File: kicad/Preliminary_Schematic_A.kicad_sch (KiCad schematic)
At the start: 5 parts, among them M1 Motor_Servo, U2 40PC015G, U3 TSSP58038

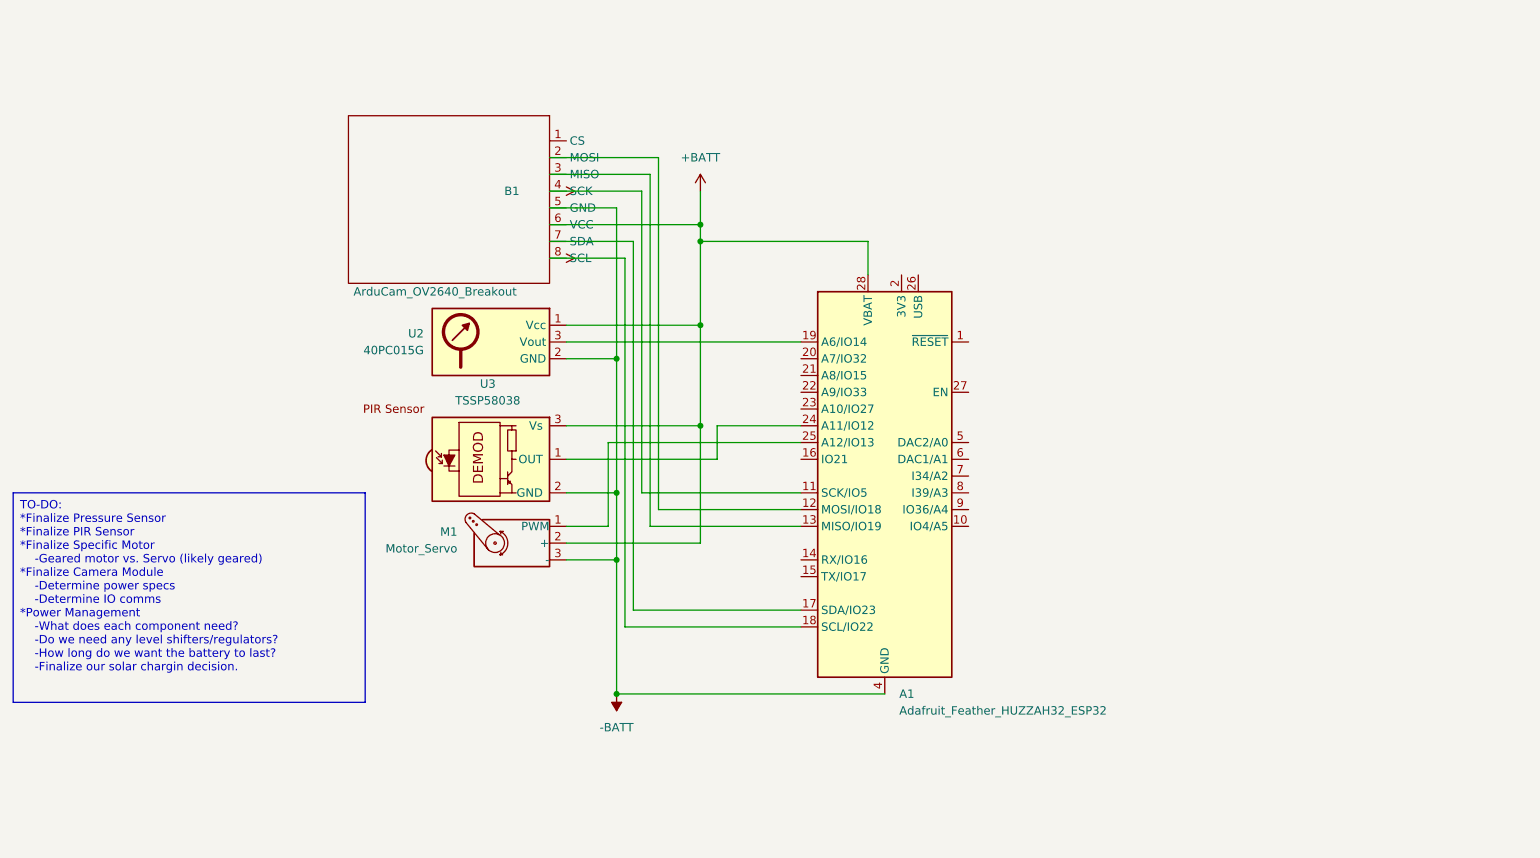
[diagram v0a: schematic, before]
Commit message: Add files via upload
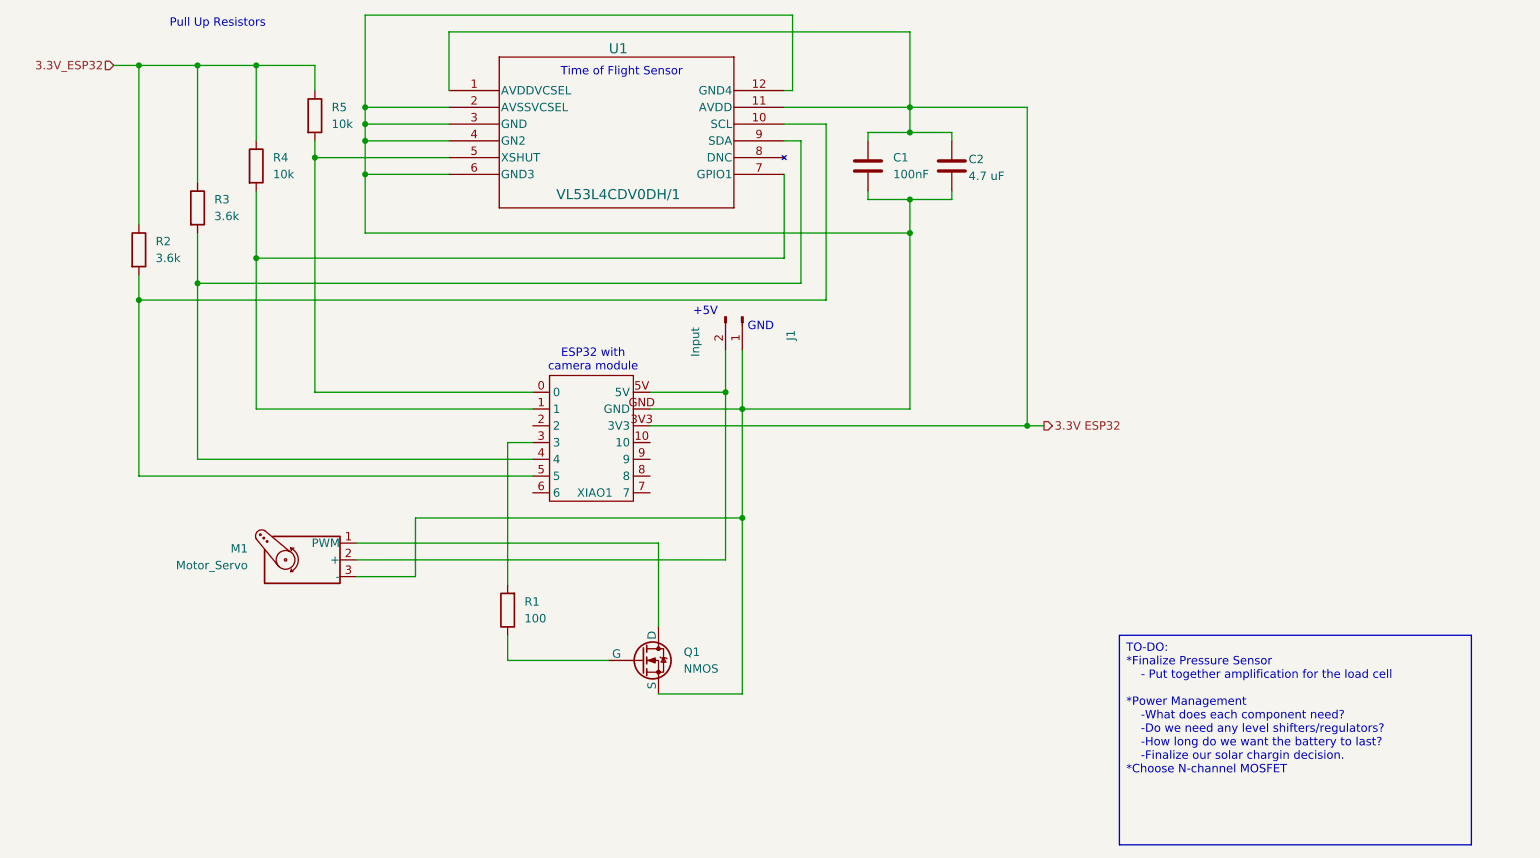
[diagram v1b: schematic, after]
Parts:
- removed A1: Adafruit_Feather_HUZZAH32_ESP32, Module:Adafruit_Feather, symbol MCU_Module:Adafruit_Feather_HUZZAH32_ESP32
- removed B1: ArduCam_OV2640_Breakout, symbol symbols:ArduCam_OV2640_Breakout
- removed U2: 40PC015G, symbol Sensor_Pressure:40PC015G
- removed U3: TSSP58038, OptoDevice:Vishay_MINICAST-3Pin, symbol Sensor_Proximity:TSSP58038
- added C1: 100nF, Capacitor_SMD:C_0805_2012Metric_Pad1.18x1.45mm_HandSolder, symbol Device:C
- added C2: 4.7 uF, Capacitor_SMD:C_0805_2012Metric_Pad1.18x1.45mm_HandSolder, symbol Device:C
- added J1: Input, Connector_PinHeader_2.54mm:PinHeader_1x02_P2.54mm_Vertical, symbol Connector:Conn_01x02_Pin
- added Q1: NMOS, symbol Simulation_SPICE:NMOS
- added R1: 100, Resistor_SMD:R_0805_2012Metric_Pad1.20x1.40mm_HandSolder, symbol Device:R
- added R2, R3: 3.6k, Resistor_SMD:R_0805_2012Metric_Pad1.20x1.40mm_HandSolder, symbol Device:R
- added R4, R5: 10k, Resistor_SMD:R_0805_2012Metric_Pad1.20x1.40mm_HandSolder, symbol Device:R
- added U1: VL53L4CDV0DH/1, LGA12_STM, symbol 2024-11-07_06-19-20:VL53L4CDV0DH_1
- added XIAO1: ~, Dev_boards:XIAO_QTpy, symbol XIAO:esp32s3
- M1: footprint (none) -> Connector_PinHeader_2.54mm:PinHeader_1x03_P2.54mm_Vertical
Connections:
- net at M1.1 (PWM): now also Q1.1 (D)
- net +BATT: no longer names the net of M1.2 (+)
- net +BATT: now also J1.2 (Pin_2), XIAO1.5V
- net -BATT: no longer names the net of M1.3 (-)
- net -BATT: now also C1.2, C2.2, J1.1 (Pin_1), Q1.3 (S), U1.12 (GND4), U1.2 (AVSSVCSEL), U1.3 (GND), U1.4 (GN2), U1.6 (GND3), XIAO1.GND
- new net: R2.2, U1.10 (SCL), XIAO1.5
- new net: Q1.2 (G), R1.1
- new net: R5.2, U1.5 (XSHUT), XIAO1.0
- new net: R4.2, U1.7 (GPIO1), XIAO1.1
- new net: R1.2, XIAO1.3
- new net: R3.2, U1.9 (SDA), XIAO1.4
- new net 3.3V ESP32: C1.1, C2.1, U1.1 (AVDDVCSEL), U1.11 (AVDD), XIAO1.3V3
- new net 3.3V_ESP32: R2.1, R3.1, R4.1, R5.1
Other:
- note added: "+5V"
- note added: "ESP32 with camera module"
- note added: "GND"
- note added: "Pull Up Resistors"
- note added: "Time of Flight Sensor"
- moved on the sheet: M1
